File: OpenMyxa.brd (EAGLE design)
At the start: 56 x 56 mm, 107 parts, among them CON1 USB, CON2 PINHEAD_1X01-2, CON3 CON-4P-STRAIGHT, CON4 CON-4P-STRAIGHT, CON5 CON-4P-STRAIGHT, CON6 CON-4P-STRAIGHT, CON7 CON-4P-STRAIGHT, CON8 CON-6P, CON9 PINHEAD_1X01-2, IC1 TPD3S014DBVR-SOT23-6, IC2 TPD3S014DBVR-SOT23-6, IC3 TJA1051, IC4 TJA1051, IC5 MCP9700, Q1 BSC040N08NS5ATMA1-PG-TDSON-8-7, Q10 BSC040N08NS5ATMA1-PG-TDSON-8-7, Q11 BSC040N08NS5ATMA1-PG-TDSON-8-7, Q12 BSC040N08NS5ATMA1-PG-TDSON-8-7, Q2 BSC040N08NS5ATMA1-PG-TDSON-8-7, Q3 BSC040N08NS5ATMA1-PG-TDSON-8-7, Q4 BSC040N08NS5ATMA1-PG-TDSON-8-7, Q5 BSC040N08NS5ATMA1-PG-TDSON-8-7, Q6 BSC040N08NS5ATMA1-PG-TDSON-8-7, Q7 BSC040N08NS5ATMA1-PG-TDSON-8-7, Q8 BSC040N08NS5ATMA1-PG-TDSON-8-7, Q9 BSC040N08NS5ATMA1-PG-TDSON-8-7

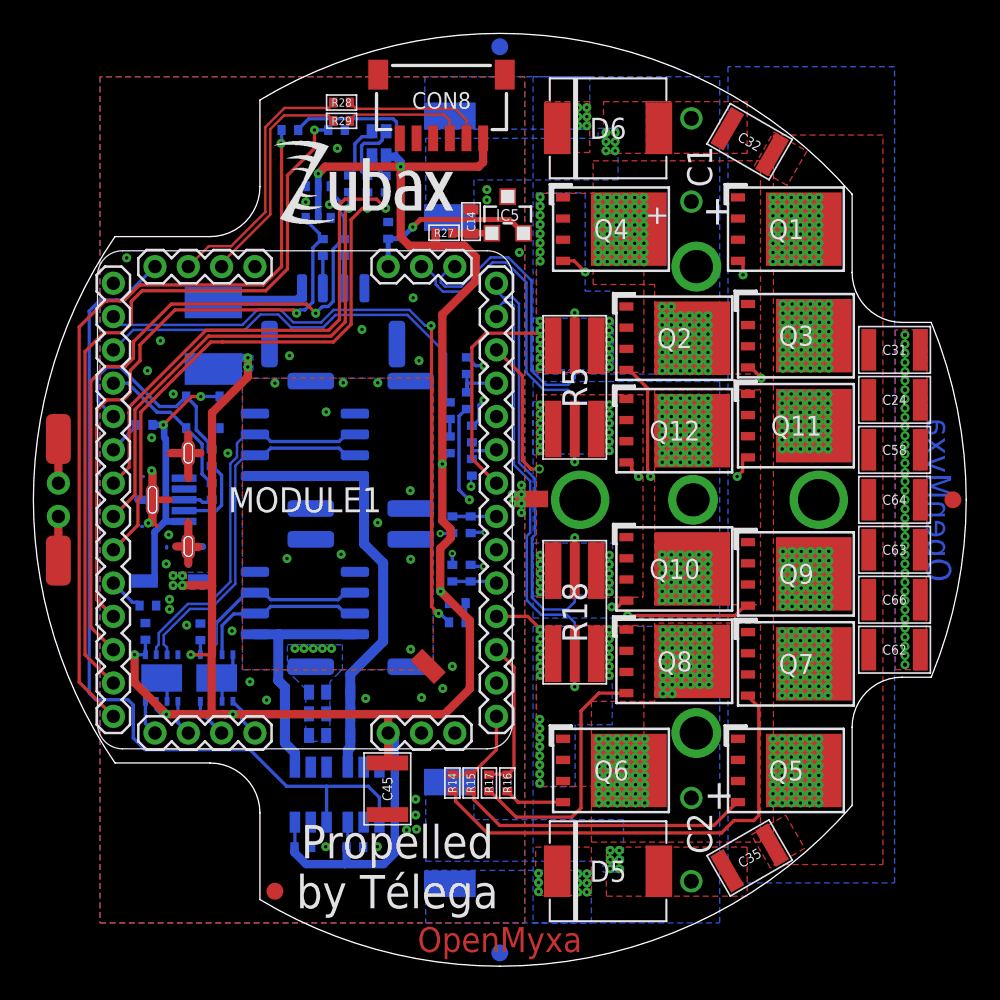
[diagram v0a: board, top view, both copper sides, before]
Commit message: V0.2 import
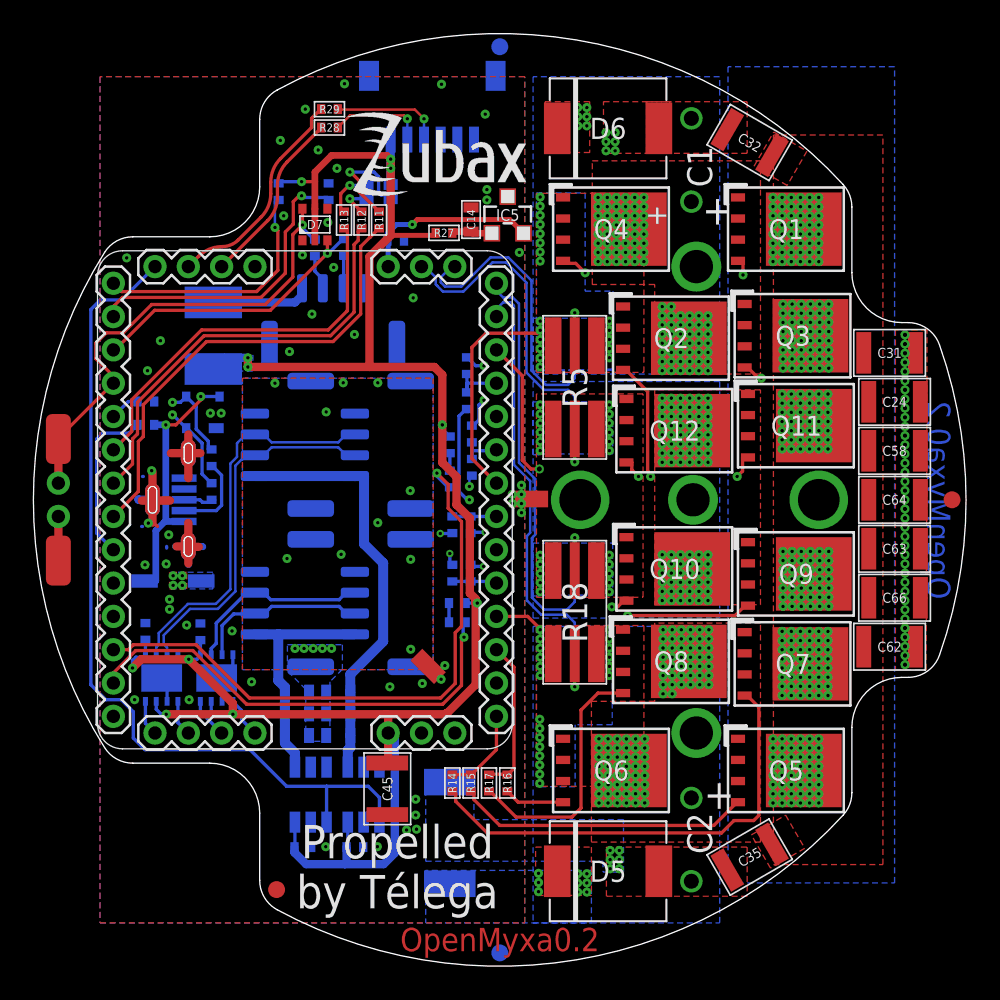
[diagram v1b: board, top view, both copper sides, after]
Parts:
- removed D3: TPSMC62A, TVS_diodes:DO-214AB(SMC)
- removed MODULE1: MITOHONDRIQUE, mitohondrique:MITOHONDRIQUE
- added MODULE2: MITOHONDRIQUE-TH, zubax_modules:MITOHONDRIQUE
- CON3, CON4, CON5, CON6: device myxa_masterlib:JST_GH-4P-STRAIGHT -> Connectors:JST_GH-4P-STRAIGHT
- moved R7 12.3 mm to (-21.2, 5.90)
- moved PAD6 7.30 mm to (-26.5, -3.65), turned to 270 degrees
- moved PAD7 7.30 mm to (-26.5, 3.65), turned to 270 degrees
- moved U$13 4.69 mm to (-9.28, 18.1)
- moved R10 4.10 mm to (-3.00, 1.25), turned to 90 degrees
- moved LED5 3.76 mm to (-13.3, 18.5), turned to 90 degrees
- moved LED4 3.73 mm to (-10.3, 18.5), turned to 270 degrees
- moved LED3 2.90 mm to (-7.28, 18.5), turned to 270 degrees
- moved R13 2.57 mm to (-9.35, 16.8), flipped to the top
- moved R12 2.30 mm to (-8.30, 16.8), flipped to the top
- moved R11 2.19 mm to (-7.25, 16.8), flipped to the top
- moved CON2 2.00 mm to (-26.5, 1.00), turned to 270 degrees
- moved CON9 2.00 mm to (-26.5, -1.00), turned to 270 degrees
- moved R28 1.67 mm to (-10.2, 22.4)
- moved D7 1.36 mm to (-11.1, 16.5), flipped to the top, turned to 90 degrees
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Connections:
- removed net N$23: CON3.2, CON4.2, IC3.6
- removed net N$24: CON7.2, R25.2
- removed net N$35: CON3.3, CON4.3, IC3.7
- new net LED_BLUE: MODULE2.32, R11.2
- new net N$21: CON3.2, CON4.2, IC3.7
- new net N$22: CON3.3, CON4.3, IC3.6
- net BEC_ENABLE_OUT: now also MODULE2.24; no longer MODULE1.24
- net CAN1_LED: now also MODULE2.36; no longer MODULE1.27
- net CAN1_RX: now also MODULE2.41; no longer MODULE1.41
- net CAN1_TX: now also MODULE2.42; no longer MODULE1.42
- net CAN1_VDD: now also CON3.1, CON4.1; no longer CON3.4, CON4.4
- net CAN2_LED: now also MODULE2.37; no longer MODULE1.26
- net CAN2_RX: now also MODULE2.39; no longer MODULE1.39
- net CAN2_TX: now also MODULE2.40; no longer MODULE1.40
- net CAN2_VDD: now also CON5.1, CON6.1; no longer CON5.4, CON6.4
- net GAIN_OUT: now also MODULE2.25; no longer MODULE1.38
- net GATE_ENABLE_OUT: now also MODULE2.26; no longer MODULE1.37
- net GND: now also CON7.4, MODULE2.2; no longer CON7.1, MODULE1.2
- net GNDD: now also CON3.4, CON4.4, CON5.4, CON6.4; no longer CON3.1, CON4.1, CON5.1, CON6.1
- net GPIO1: now also MODULE2.28; no longer MODULE1.35
- net GPIO2: now also MODULE2.27; no longer MODULE1.36
- net LED_GREEN: now also MODULE2.31; no longer MODULE1.32
- net LED_RED: now also MODULE2.30; no longer MODULE1.33
- net N$18: now also MODULE2.29; no longer MODULE1.34
- net N$19: now also CON7.2, R8.2; no longer CON7.4, F1.P$1
- net N$20: now also R25.2; no longer R8.2
- net N$44: now also CON5.3, CON6.3; no longer CON5.2, CON6.2
- net N$46: now also CON5.2, CON6.2; no longer CON5.3, CON6.3
- net N$5: now also MODULE2.33; no longer MODULE1.30
- net N$51: now also MODULE2.34; no longer MODULE1.29
- net N$55: now also MODULE2.35; no longer MODULE1.28
- net N$6: now also CON7.1, F1.P$1; no longer MODULE1.31, R11.2
- net PGND: no longer D3.A
- net PHASE_A: now also MODULE2.5; no longer MODULE1.5
- net PHASE_A_CURRENT_SHUNT_N: now also MODULE2.16; no longer MODULE1.16
- net PHASE_A_CURRENT_SHUNT_P: now also MODULE2.17; no longer MODULE1.17
- net PHASE_A_GATE_HIGH: now also MODULE2.4; no longer MODULE1.4
- net PHASE_A_GATE_LOW: now also MODULE2.6; no longer MODULE1.6
- net PHASE_A_GND: now also MODULE2.7; no longer MODULE1.7
- net PHASE_B: now also MODULE2.9; no longer MODULE1.9
- net PHASE_B_CURRENT_SHUNT_N: now also MODULE2.18; no longer MODULE1.18
- net PHASE_B_CURRENT_SHUNT_P: now also MODULE2.19; no longer MODULE1.19
- net PHASE_B_GATE_HIGH: now also MODULE2.8; no longer MODULE1.8
- net PHASE_B_GATE_LOW: now also MODULE2.10; no longer MODULE1.10
- net PHASE_B_GND: now also MODULE2.11; no longer MODULE1.11
- net PHASE_C: now also MODULE2.13; no longer MODULE1.13
- net PHASE_C_GATE_HIGH: now also MODULE2.12; no longer MODULE1.12
- net PHASE_C_GATE_LOW: now also MODULE2.14; no longer MODULE1.14
- net PHASE_C_GND: now also MODULE2.15; no longer MODULE1.15
- net TEMPERATURE_SENSOR: now also MODULE2.20; no longer MODULE1.20
- net UART_RX: now also MODULE2.23, R29.2; no longer MODULE1.23, R28.2
- net UART_TX: now also MODULE2.22, R28.2; no longer MODULE1.22, R29.2
- net VDC: now also MODULE2.3; no longer D3.C, MODULE1.3
- net VDD_5V: now also MODULE2.1; no longer MODULE1.1
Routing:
- net GAIN_OUT: track 46.1 -> 15.0 mm
- net LED_BLUE: track 0.00 -> 28.4 mm
- net GATE_ENABLE_OUT: track 45.4 -> 18.6 mm
- net N$6: track 30.7 -> 5.93 mm, vias 1 -> 0
- net GPIO2: track 41.8 -> 17.4 mm
- net GPIO1: track 45.7 -> 29.2 mm
- net CAN1_LED: track 25.5 -> 37.0 mm, vias 0 -> 1
- net N$23: track 11.5 -> 0.00 mm
- net N$22: track 0.00 -> 11.5 mm
- net CAN2_LED: track 39.0 -> 27.8 mm, vias 2 -> 1
- net N$35: track 10.4 -> 0.00 mm
- net N$21: track 0.00 -> 10.4 mm
- net N$55: track 9.44 -> 19.1 mm, vias 0 -> 1
- net LED_RED: track 32.3 -> 23.7 mm, vias 1 -> 0
- net N$5: track 2.09 -> 9.95 mm
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- added copper zone on layer 15, net VDD_5V
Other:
- outline, holes or cut-outs redrawn
- board text added: "OpenMyxa0.2"
- board text removed: "OpenMyxa"
